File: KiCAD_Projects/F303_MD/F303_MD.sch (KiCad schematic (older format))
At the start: 12 parts, among them P1 CONN_01X06, P2 CONN_01X06, SW1 SW_PUSH, U1 STM32F303K8, X1 CRYSTAL

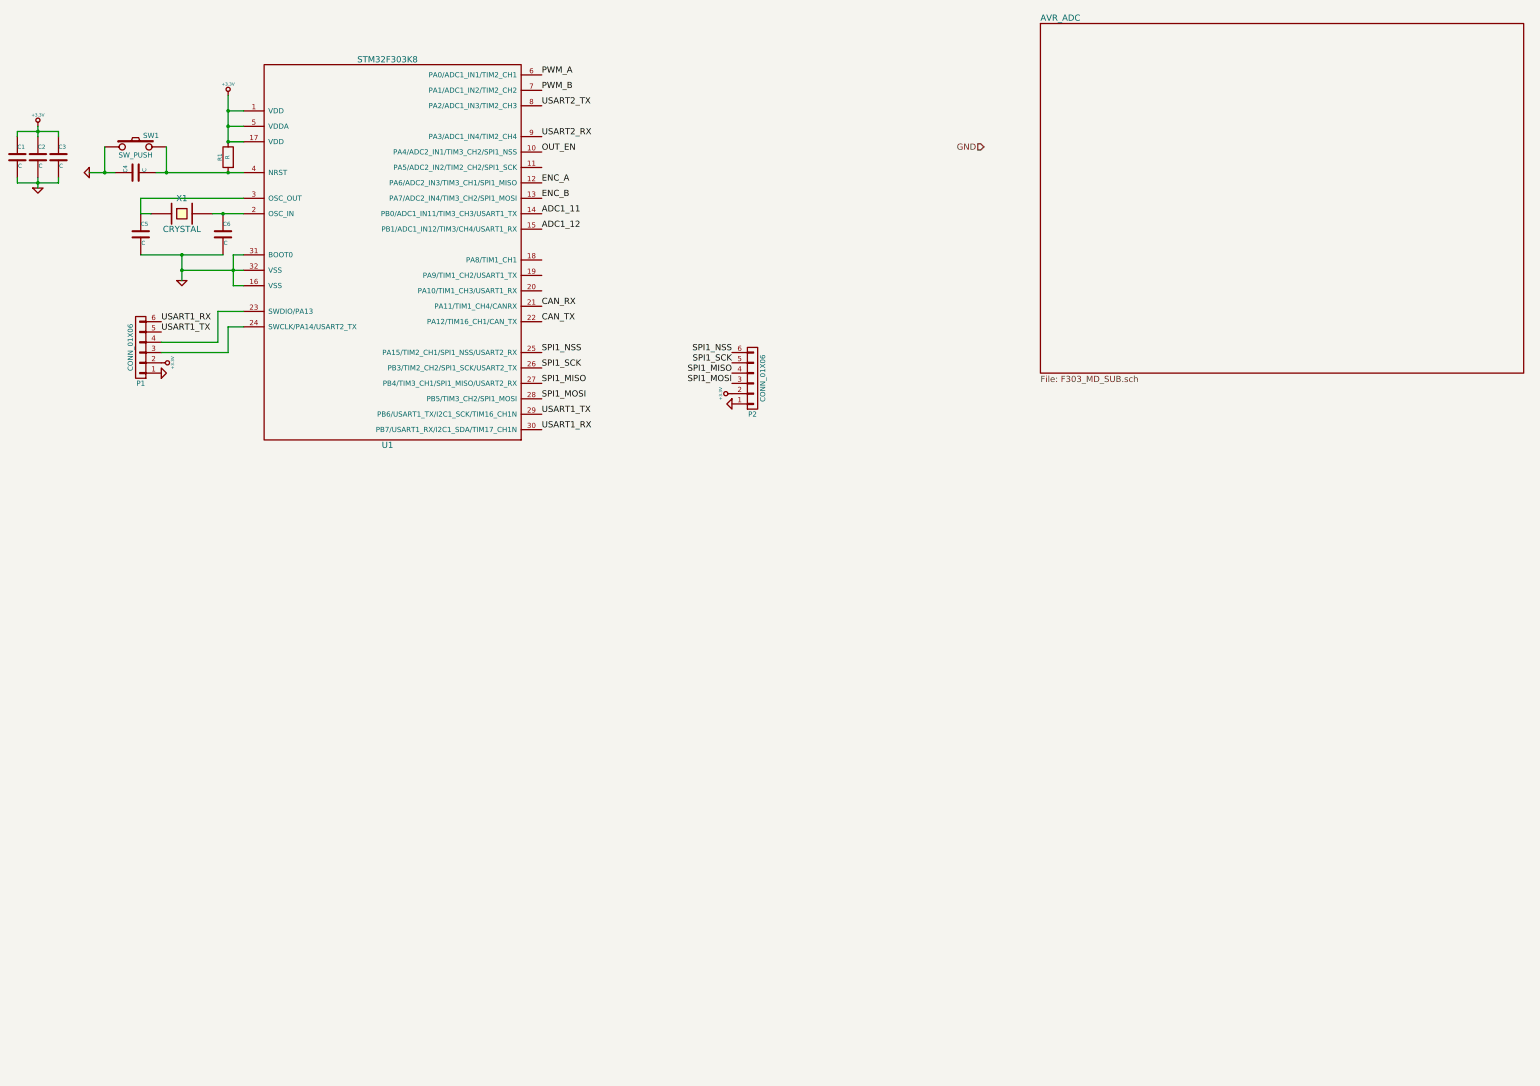
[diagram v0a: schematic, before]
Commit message: no message
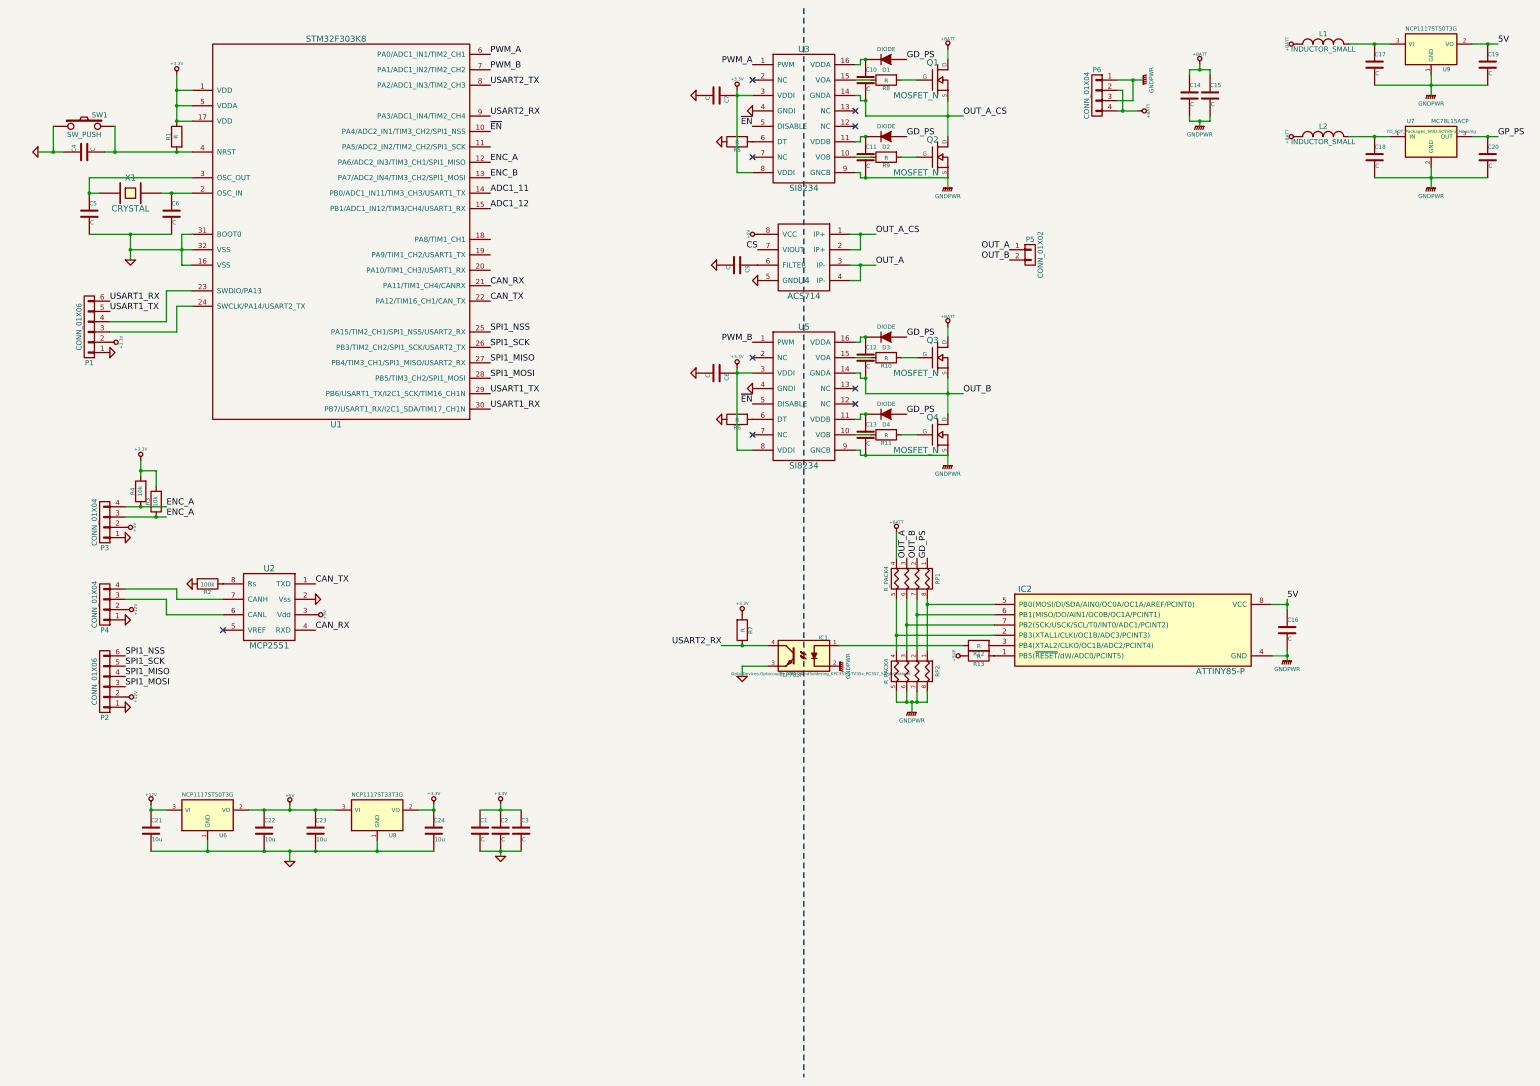
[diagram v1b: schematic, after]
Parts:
- added C10, C11, C12, C13: C, RP_KiCAD_Libs:C3216, symbol C
- added C14, C15: C, Capacitors_SMD:c_elec_10x10.5, symbol C
- added C16, C7, C8, C9: C, RP_KiCAD_Libs:C1608, symbol C
- added C17, C18, C19, C20: C, RP_KiCAD_Libs:C2012, symbol C
- added C21, C22, C23, C24: 10u, RP_KiCAD_Libs:C2012, symbol C
- added D1, D2, D3, D4: DIODE, RP_KiCAD_Libs:C3216, symbol DIODE
- added IC1: TLP785F, Opto-Devices:Optocoupler_SMD_HandSoldering_KPC357_LTV35x_PC357_SingleChannel, symbol TLP785F
- added IC2: ATTINY85-P, Housings_SOIC:SOIC-8_3.9x4.9mm_Pitch1.27mm, symbol ATTINY85-P
- added L1, L2: INDUCTOR_SMALL, Choke_SMD:Choke_SMD_1206_Standard, symbol INDUCTOR_SMALL
- added P3, P4: CONN_01X04, RP_KiCAD_Connector:XA_4L, symbol CONN_01X04
- added P5: CONN_01X02, RP_KiCAD_Connector:D-3200S_2L, symbol CONN_01X02
- added P6: CONN_01X04, RP_KiCAD_Connector:D-3500D_4S, symbol CONN_01X04
- added Q1, Q2, Q3, Q4: MOSFET_N, TO_SOT_Packages_SMD:D2-PAK, symbol MOSFET_N
- added R10, R11, R12, R13, R5, R6, R7, R8, R9: R, RP_KiCAD_Libs:C1608, symbol R
- added R2: 100k, RP_KiCAD_Libs:C1608, symbol R
- added R3, R4: 10k, RP_KiCAD_Libs:C1608, symbol R
- added RP1, RP2: R_PACK4, Resistors_SMD:R_Array_Convex_4x0603, symbol R_PACK4
- added U2: MCP2551, Housings_SOIC:SOIC-8_3.9x4.9mm_Pitch1.27mm, symbol MCP2551
- added U3, U5: SI8234, Housings_SOIC:SOIC-16_3.9x9.9mm_Pitch1.27mm, symbol SI8234
- added U4: ACS714, Housings_SOIC:SOIC-8_3.9x4.9mm_Pitch1.27mm, symbol ACS714
- added U6, U9: NCP1117ST50T3G, TO_SOT_Packages_SMD:SOT89-3_Housing, symbol NCP1117ST50T3G
- added U7: MC78L15ACP, TO_SOT_Packages_SMD:SOT89-3_Housing, symbol MC78L15ACP
- added U8: NCP1117ST33T3G, TO_SOT_Packages_SMD:SOT89-3_Housing, symbol NCP1117ST33T3G
- P1, P2: footprint (none) -> RP_KiCAD_Connector:XA_6T
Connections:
- net +3.3V: now also C24.1, C7.1, C8.1, R3.1, R4.1, R7.1, U3.3 (VDDI), U3.8 (VDDI), U5.3 (VDDI), U5.8 (VDDI), U8.2 (VO); no longer P2.2 (P2)
- net CAN_RX: now also U2.4 (RXD)
- net CAN_TX: now also U2.1 (TXD)
- net ENC_A: now also P3.3 (P3), P3.4 (P4), R3.2, R4.2
- net GND: now also C21.2, C22.2, C23.2, C24.2, C7.2, C8.2, C9.2, IC1.3, P3.1 (P1), P4.1 (P1), R2.1, R5.2, R6.2, U2.2 (Vss), U3.4 (GNDI), U4.5 (GND), U5.4 (GNDI), U6.1 (GND), U8.1 (GND)
- net PWM_A: now also U3.1 (PWM)
- net PWM_B: now also U5.1 (PWM)
- net USART2_RX: now also IC1.4, R7.2
- net OUT_EN renamed ~EN
- net ~EN: now also U3.5 (DISABLE), U5.5 (DISABLE)
- new net: Q1.G, R8.1
- new net: Q2.G, R9.1
- new net: C9.1, U4.6 (FILTER)
- new net: R9.2, U3.10 (VOB)
- new net: C11.1, D2.2 (K), U3.11 (VDDB)
- new net: R8.2, U3.15 (VOA)
- new net: C10.1, D1.2 (K), U3.16 (VDDA)
- new net: R5.1, U3.6 (DT)
- new net: Q3.G, R10.1
- new net: Q4.G, R11.1
- new net: R11.2, U5.10 (VOB)
- new net: C13.1, D4.2 (K), U5.11 (VDDB)
- new net: R10.2, U5.15 (VOA)
- new net: C12.1, D3.2 (K), U5.16 (VDDA)
- new net: R6.1, U5.6 (DT)
- new net: C17.1, L1.2, U9.3 (VI)
- new net: P4.3 (P3), U2.6 (CANL)
- new net: P4.4 (P4), U2.7 (CANH)
- new net: R2.2, U2.8 (Rs)
- new net: IC2.1 (PB5(~RESET~/dW/ADC0/PCINT5)), R13.1
- new net: IC2.2 (PB3(XTAL1/CLKI/OC1B/ADC3/PCINT3)), RP1.5 (R4), RP2.4 (P4)
- new net: IC2.3 (PB4(XTAL2/CLKO/OC1B/ADC2/PCINT4)), R12.1
- new net: IC2.5 (PB0(MOSI/DI/SDA/AIN0/OC0A/OC1A/AREF/PCINT0)), RP1.8 (R1), RP2.1 (P1)
- new net: IC2.6 (PB1(MISO/DO/AIN1/OC0B/OC1A/PCINT1)), RP1.7 (R2), RP2.2 (P2)
- new net: IC2.7 (PB2(SCK/USCK/SCL/T0/INT0/ADC1/PCINT2)), RP1.6 (R3), RP2.3 (P3)
- new net: IC1.1, R12.2
- new net: C18.1, L2.2, U7.1 (IN)
- new net +12V: C21.1, P2.2 (P2), P4.2 (P2), U6.3 (VI)
- new net +5V: C22.1, C23.1, P3.2 (P2), U2.3 (Vdd), U4.8 (VCC), U6.2 (VO), U8.3 (VI)
- new net +5VP: R13.2
- new net +BATT: C14.1, C15.1, L1.1, L2.1, P6.2 (P2), P6.4 (P4), Q1.D, Q3.D, RP1.4 (P4)
- new net 5V: C16.1, C19.1, IC2.8 (VCC), U9.2 (VO)
- new net CS: U4.7 (VIOUT)
- new net GD_PS: D1.1 (A), D2.1 (A), D3.1 (A), D4.1 (A), RP1.1 (P1)
- new net GNDPWR: C11.2, C13.2, C14.2, C15.2, C16.2, C17.2, C18.2, C19.2, C20.2, IC1.2, IC2.4 (GND), P6.1 (P1), P6.3 (P3), Q2.S, Q4.S, RP2.5 (R4), RP2.6 (R3), RP2.7 (R2), RP2.8 (R1), U3.9 (GNCB), U5.9 (GNCB), U7.2 (GND), U9.1 (GND)
- new net GP_PS: C20.1, U7.3 (OUT)
- new net OUT_A: P5.1 (P1), RP1.3 (P3), U4.3 (IP-), U4.4 (IP-)
- new net OUT_A_CS: C10.2, Q1.S, Q2.D, U3.14 (GNDA), U4.1 (IP+), U4.2 (IP+)
- new net OUT_B: C12.2, P5.2 (P2), Q3.S, Q4.D, RP1.2 (P2), U5.14 (GNDA)
- no-connect marks 0 -> 9
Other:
- moved on the sheet: C1, C2, C3, C4, C5, C6, P1, P2, R1, SW1, U1, X1
